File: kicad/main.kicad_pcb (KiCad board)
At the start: 2 copper layers, 190.5 x 97.2 mm, 71 parts, among them J1 Jack-DC, J10 RS232, J11 UART, J12 I2C1, J13 I2C2, J2 LCD_Conn, J3 Data, J4 PWR, J5 uSD, J6 VIA_B, J7 IO~{EN}_{[2..7]}, J8 Control, J9 Addr, P1 Mini-DIN-6, SW1 Step, SW2 Reset, U1 74HC00, U2 74HC00, U3 MAX232, U4 DS1307N+, U5 MCP9808_MSOP, X1 4 MHz, X2 1.8432 MHz, Y1 32.768 KHz

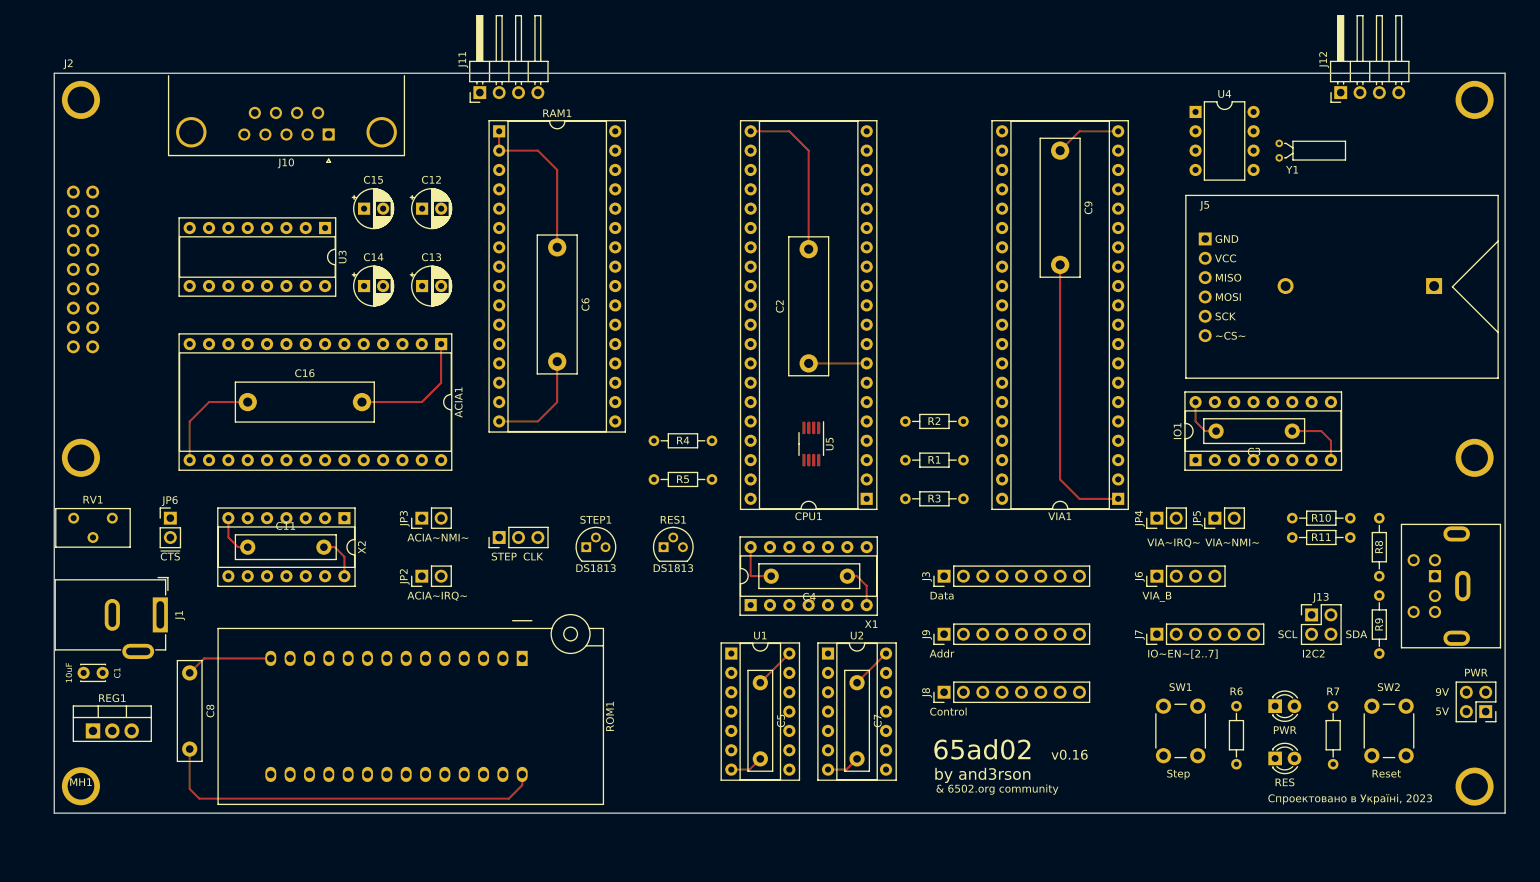
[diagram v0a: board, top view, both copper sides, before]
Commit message: WIP: V16
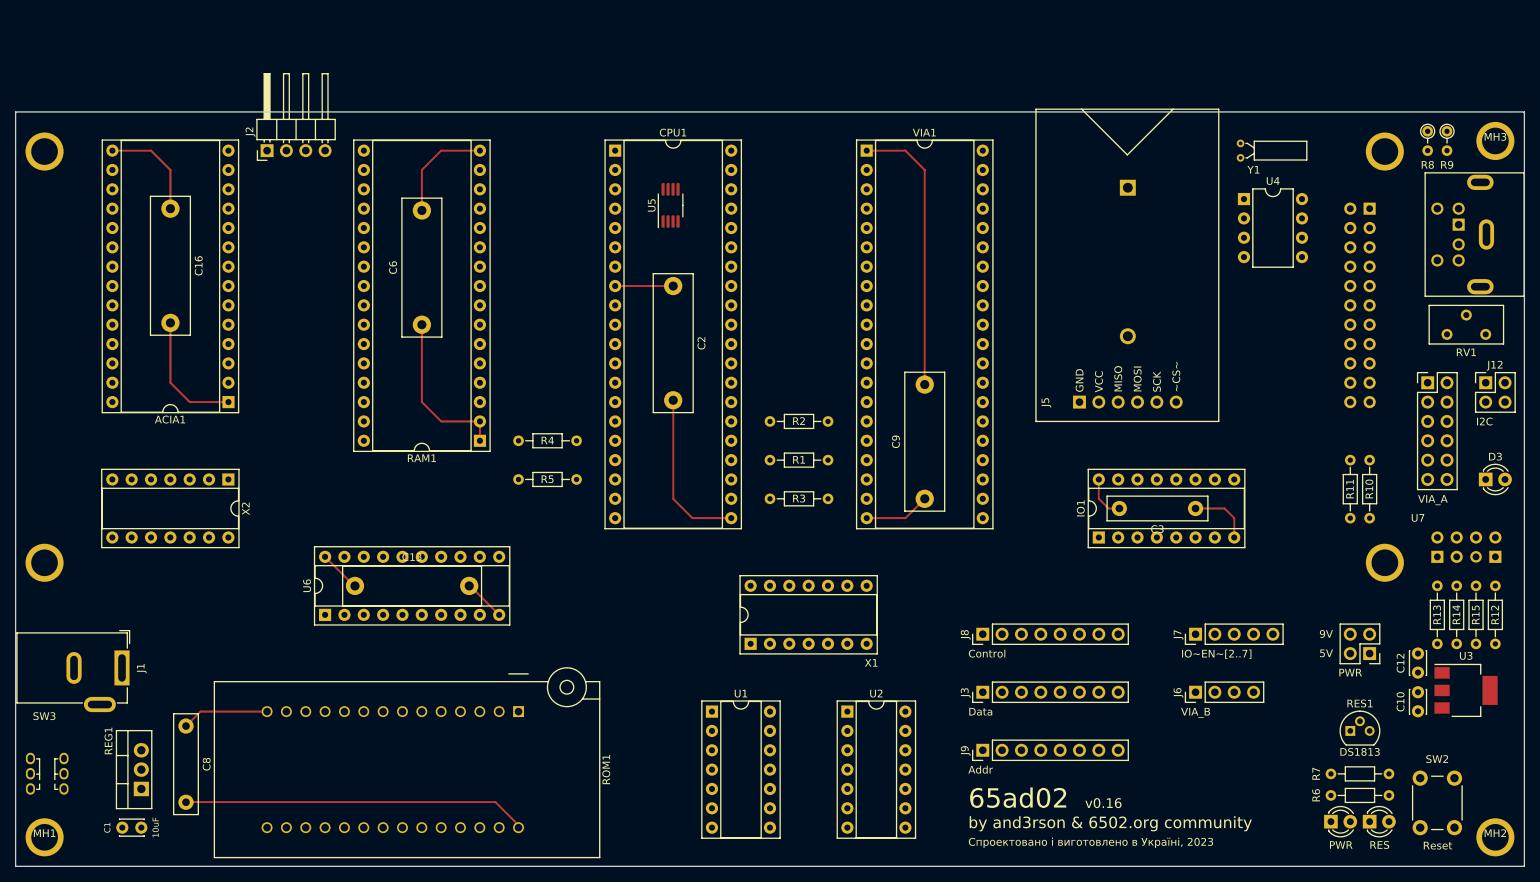
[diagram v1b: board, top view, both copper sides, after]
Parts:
- removed C11, C4: 0,1uF, Capacitor_THT:C_Rect_L13.0mm_W3.0mm_P10.00mm_FKS3_FKP3_MKS4
- removed C14, C15: 10uF, Capacitor_THT:CP_Radial_D5.0mm_P2.50mm
- removed C5, C7: 0.1uF, Capacitor_THT:C_Rect_L13.0mm_W3.0mm_P10.00mm_FKS3_FKP3_MKS4
- removed J10: RS232, Connector_Dsub:DSUB-9_Male_Horizontal_P2.77x2.84mm_EdgePinOffset4.94mm_Housed_MountingHolesOffset7.48mm
- removed J11: UART, Connector_PinHeader_2.54mm:PinHeader_1x04_P2.54mm_Horizontal
- removed J13: I2C2, Connector_PinHeader_2.54mm:PinHeader_2x02_P2.54mm_Vertical
- removed JP1: Clock_Mode, Connector_PinHeader_2.54mm:PinHeader_1x03_P2.54mm_Vertical
- removed JP2: ACIA~{IRQ}, Connector_PinHeader_2.54mm:PinHeader_1x02_P2.54mm_Vertical
- removed JP3: ACIA~{NMI}, Connector_PinHeader_2.54mm:PinHeader_1x02_P2.54mm_Vertical
- removed JP4: VIA~{IRQ}, Connector_PinHeader_2.54mm:PinHeader_1x02_P2.54mm_Vertical
- removed JP5: VIA~{NMI}, Connector_PinHeader_2.54mm:PinHeader_1x02_P2.54mm_Vertical
- removed JP6: ~{CTS}, Connector_PinHeader_2.54mm:PinHeader_1x02_P2.54mm_Vertical
- removed STEP1: DS1813, Package_TO_SOT_THT:TO-92
- removed SW1: Step, Button_Switch_THT:SW_PUSH_6mm_H5mm
- added C10: 10uF, Capacitor_THT:C_Disc_D3.0mm_W2.0mm_P2.50mm, F.Cu at (199.4, 101.6)
- added D3: DATA, LED_THT:LED_D3.0mm, F.Cu at (208.3, 71.1)
- added J14: LCD_Conn, my:LCD24064, F.Cu at (17.0, 22.6)
- added J15: VIA_A, Connector_PinHeader_2.54mm:PinHeader_2x06_P2.54mm_Vertical, F.Cu at (200.7, 58.4)
- added MH3: MountingHole, my:Hole_3.5x5, F.Cu at (209.6, 26.7)
- added R12: 300, Resistor_THT:R_Axial_DIN0204_L3.6mm_D1.6mm_P7.62mm_Horizontal, F.Cu at (209.6, 92.7)
- added R13: 10K, Resistor_THT:R_Axial_DIN0204_L3.6mm_D1.6mm_P7.62mm_Horizontal, F.Cu at (201.9, 85.1)
- added R14: 10K, Resistor_THT:R_Axial_DIN0204_L3.6mm_D1.6mm_P7.62mm_Horizontal, F.Cu at (204.5, 85.1)
- added R15: 10K, Resistor_THT:R_Axial_DIN0204_L3.6mm_D1.6mm_P7.62mm_Horizontal, F.Cu at (207.0, 85.1)
- added SW3: SW_PWR, my:PB22E06, F.Cu at (16.5, 106.9)
- added U6: GAL16V8, Package_DIP:DIP-20_W7.62mm_Socket, F.Cu at (55.9, 88.9)
- added U7: ESP-01, my:ESP-01, F.Cu at (205.7, 77.5)
- C12: value 10uF -> 22uF; footprint Capacitor_THT:CP_Radial_D5.0mm_P2.50mm -> Capacitor_THT:C_Disc_D3.0mm_W2.0mm_P2.50mm
- C13: value 10uF -> 0.1uF; footprint Capacitor_THT:CP_Radial_D5.0mm_P2.50mm -> Capacitor_THT:C_Rect_L18.0mm_W5.0mm_P15.00mm_FKS3_FKP3
- J12: footprint Connector_PinHeader_2.54mm:PinHeader_1x04_P2.54mm_Horizontal -> Connector_PinHeader_2.54mm:PinHeader_2x02_P2.54mm_Vertical
- J2: value LCD_Conn -> UART; footprint my:LCD_4004 -> Connector_PinHeader_2.54mm:PinHeader_1x04_P2.54mm_Horizontal
- J7: value IO~{EN}_{[2..7]} -> IO~{EN}_{[3..7]}; footprint Connector_PinHeader_2.54mm:PinHeader_1x06_P2.54mm_Vertical -> Connector_PinHeader_2.54mm:PinHeader_1x05_P2.54mm_Vertical
- R8, R9: footprint Resistor_THT:R_Axial_DIN0204_L3.6mm_D1.6mm_P7.62mm_Horizontal -> Resistor_THT:R_Axial_DIN0204_L3.6mm_D1.6mm_P2.54mm_Vertical
- U3: value MAX232 -> AMS1117; footprint Package_DIP:DIP-16_W7.62mm_Socket -> Package_TO_SOT_SMD:SOT-223-3_TabPin2
- X1: value 4 MHz -> 16 MHz
- moved RV1 176.9 mm to (203.2, 52.1), turned to 180 degrees
- moved U3 161.7 mm to (205.7, 98.8), turned to 0 degrees
- moved C12 144.3 mm to (199.4, 96.5), turned to 90 degrees
- moved RES1 93.3 mm to (190.5, 104.1)
- moved R9 61.6 mm to (203.2, 25.4)
- moved R8 58.8 mm to (200.7, 25.4), turned to -90 degrees
- moved CPU1 56.4 mm to (94.0, 27.9), turned to 0 degrees
- moved VIA1 56.4 mm to (127.0, 27.9), turned to 0 degrees
- moved C9 49.1 mm to (134.6, 73.7), turned to 90 degrees
- moved P1 46.3 mm to (204.7, 37.7)
- moved BT1 43.5 mm to (161.3, 31.8), turned to -90 degrees
- moved J12 42.6 mm to (208.3, 58.4), turned to 0 degrees
- moved RAM1 40.7 mm to (76.2, 66.0), turned to 180 degrees
- moved C13 40.4 mm to (59.8, 85.1)
- moved U5 36.4 mm to (101.2, 35.1), turned to 90 degrees
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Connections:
- ACIA1 pad 10: Net-(ACIA1-TxD) -> TX
- ACIA1 pad 12: Net-(ACIA1-RxD) -> RX
- ACIA1 pad 26: Net-(ACIA1-~{IRQ}) -> ~{IRQ}
- ACIA1 pad 8: Net-(ACIA1-~{RTS}) -> unconnected-(ACIA1-~{RTS}-Pad8)
- ACIA1 pad 9: Net-(ACIA1-~{CTS}) -> GND
- C12 pad 1: Net-(U3-C2+) -> +3.3V
- C12 pad 2: Net-(U3-C2-) -> GND
- C13 pad 1: Net-(U3-C1+) -> +5V
- C13 pad 2: Net-(U3-C1-) -> GND
- CPU1 pad 37: Ф2 -> PHV
- IO1 pad 13: IO~{EN}_{2} -> LCD~{EN}
- J1 pad 1: +9V -> Net-(J1-Pad1)
- J1 pad 2: GND -> Net-(J1-Pad2)
- J2 pad 1: LCDD7 -> GND
- J2 pad 2: LCDD6 -> +5V
- J2 pad 3: LCDD5 -> TX
- J2 pad 4: LCDD4 -> RX
- J7 pad 1: IO~{EN}_{2} -> IO~{EN}_{3}
- J7 pad 2: IO~{EN}_{3} -> IO~{EN}_{4}
- J7 pad 3: IO~{EN}_{4} -> IO~{EN}_{5}
- J7 pad 4: IO~{EN}_{5} -> IO~{EN}_{6}
- J7 pad 5: IO~{EN}_{6} -> IO~{EN}_{7}
- RV1 pad 1: GND -> +5V
- RV1 pad 2: Net-(J2-Pin_12) -> Net-(J14-Pin_4)
- RV1 pad 3: +5V -> Net-(J14-Pin_20)
- U3 pad 1: Net-(U3-C1+) -> GND
- U3 pad 2: Net-(U3-VS+) -> +3.3V
- U3 pad 3: Net-(U3-C1-) -> +5V
- VIA1 pad 2: LCDD4 -> Net-(J15-Pin_3)
- VIA1 pad 21: Net-(JP4-B) -> ~{IRQ}
- VIA1 pad 3: LCDD5 -> Net-(J15-Pin_4)
- VIA1 pad 39: unconnected-(VIA1-CA2-Pad39) -> Net-(J15-Pin_12)
- VIA1 pad 4: LCDD6 -> Net-(J15-Pin_5)
- VIA1 pad 40: unconnected-(VIA1-CA1-Pad40) -> Net-(J15-Pin_11)
- VIA1 pad 5: LCDD7 -> Net-(J15-Pin_6)
- VIA1 pad 6: LCDEN1 -> Net-(J15-Pin_7)
- VIA1 pad 7: LCDEN2 -> Net-(J15-Pin_8)
- VIA1 pad 8: LCDR~{W} -> Net-(J15-Pin_9)
- VIA1 pad 9: LCDRS -> Net-(J15-Pin_10)
- X1 pad 8: CLK -> Net-(U6-I1/CLK)
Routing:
- net +5V: track 131.8 -> 108.0 mm
- net GND: track 128.5 -> 114.0 mm
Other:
- board size 190.5 x 97.2 mm -> 198.1 x 99.1 mm
- board text added: "I2C"
- board text added: "VIA_A"
- board text added: "by and3rson & 6502.org community"
- board text added: "Спроектовано і виготовлено в Україні, 2023"
- board text removed: "& 6502.org community"
- board text removed: "ACIA~IRQ~"
- board text removed: "ACIA~NMI~"
- board text removed: "I2C2"
- board text removed: "SCL"
- board text removed: "SDA"
- board text removed: "Step"
- board text removed: "VIA~IRQ~"
- board text removed: "VIA~NMI~"
- board text removed: "by and3rson"
- board text removed: "Спроектовано в Україні, 2023"
